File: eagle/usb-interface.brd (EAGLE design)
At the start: 18 parts

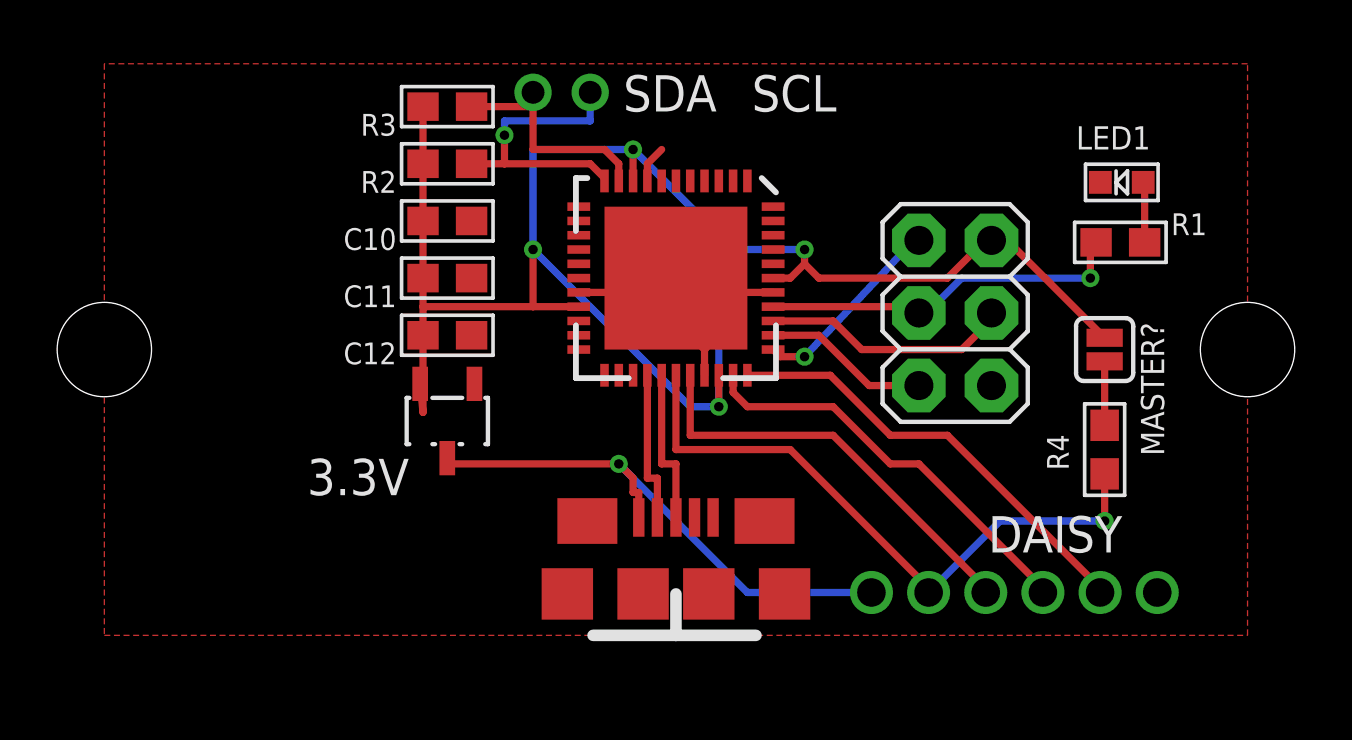
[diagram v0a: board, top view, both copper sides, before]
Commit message: major rework of usb interface board - dropped Y by 5mm, cleaned routing, added better mounting.
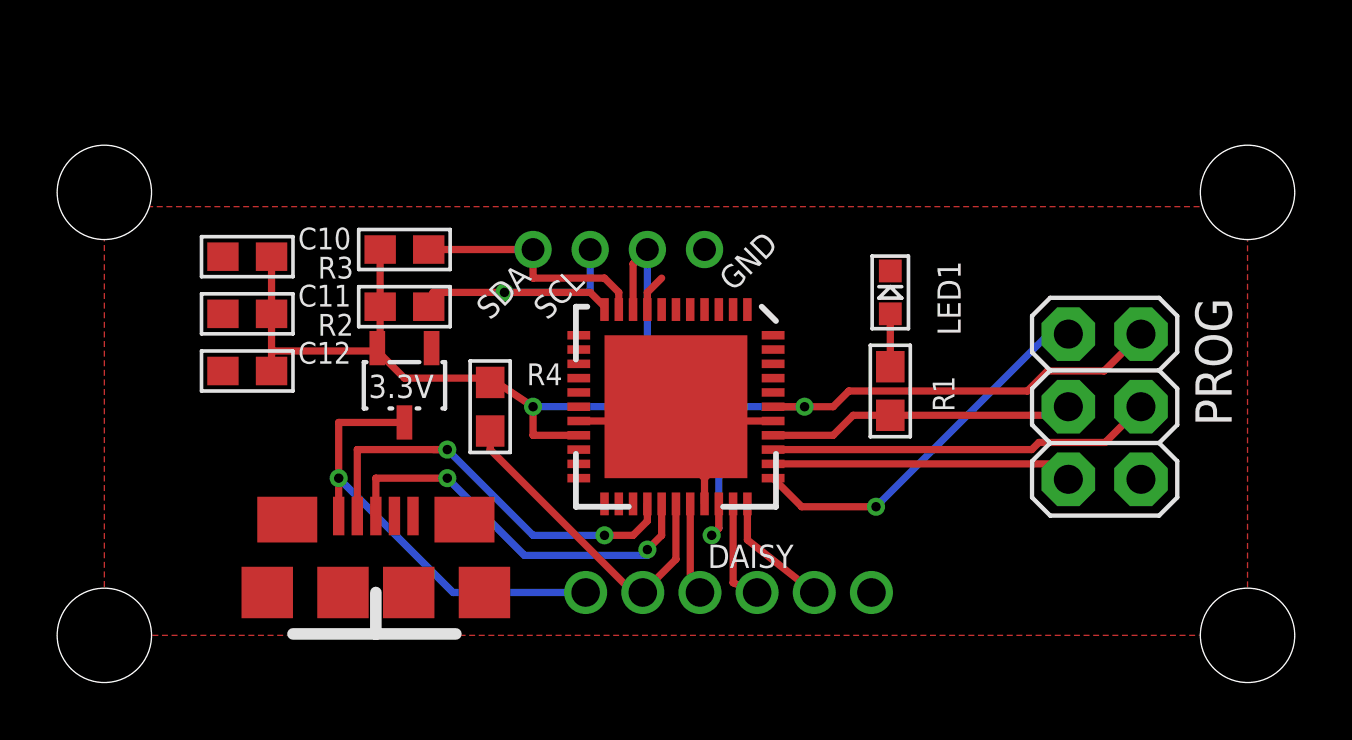
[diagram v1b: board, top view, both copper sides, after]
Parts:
- removed MASTER?: SOLDERJUMPERN, SparkFun:SJ_2S
- added JP1, JP2: (no value), nonolith:1X01_2MM
- added U$3, U$4: (no value), nonolith:STAND-OFF
- moved R4 21.6 mm to (-6.50, 8.00)
- moved CN1 10.5 mm to (-10.5, 1.50)
- moved DAISY 10.0 mm to (7.00, 1.50)
- moved U$1 10.0 mm to (-20.0, 0.00)
- moved U$2 10.0 mm to (20.0, 0.00)
- moved R1 9.58 mm to (7.50, 8.55), turned to 90 degrees
- moved LED1 8.97 mm to (7.50, 12.0), turned to 0 degrees
- moved C10 7.11 mm to (-15.0, 13.2), turned to 0 degrees
- moved C11 7.11 mm to (-15.0, 11.2), turned to 0 degrees
- moved C12 7.11 mm to (-15.0, 9.25), turned to 0 degrees
- moved PROG 6.17 mm to (15.0, 8.00)
- moved SCL 5.50 mm to (-3.00, 13.5)
- moved SDA 5.50 mm to (-5.00, 13.5)
- moved R2 5.22 mm to (-9.50, 11.5)
- moved R3 5.22 mm to (-9.50, 13.5)
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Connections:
- removed net PE0-PULL: MASTER?.2, R4.2
- net 3.3V: now also JP2.1, R4.2; no longer MASTER?.1
- net GND: now also JP1.1
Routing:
- net PE3: track 15.7 -> 4.24 mm
- net PE1: track 14.8 -> 3.64 mm
- net PE0: track 22.5 -> 11.6 mm, vias 1 -> 0
- net PE2: track 14.4 -> 3.67 mm
- net USB-: track 5.32 -> 15.0 mm, vias 0 -> 2
- net USB+: track 5.47 -> 14.0 mm, vias 0 -> 2
- net 3.3V: track 64.8 -> 57.4 mm, vias 4 -> 3
- net PDI-DATA: track 6.97 -> 13.2 mm
- net PDI-CLK: track 5.73 -> 10.8 mm
- net BOOTLOAD: track 8.73 -> 13.5 mm
- net 5V: track 19.2 -> 15.9 mm
- net PR1: track 13.5 -> 10.7 mm, vias 1 -> 0
- net PE0-PULL: track 2.24 -> 0.00 mm
- net SCL: track 10.5 -> 11.5 mm
- net SDA: track 7.96 -> 8.46 mm
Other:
- board text added: "GND"
- board text added: "SCL"
- board text added: "SDA"

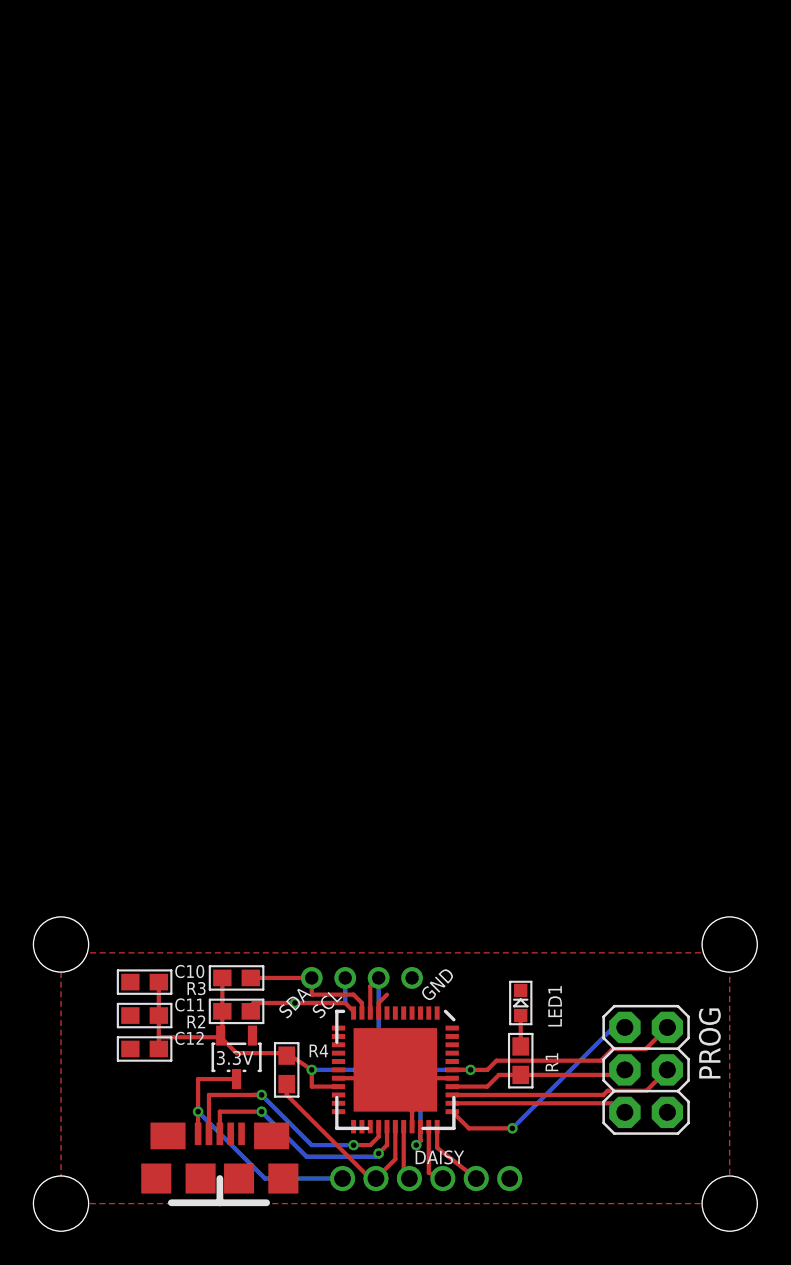
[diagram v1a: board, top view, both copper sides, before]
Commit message: reworked silkscreen and snap on tesselate.brd
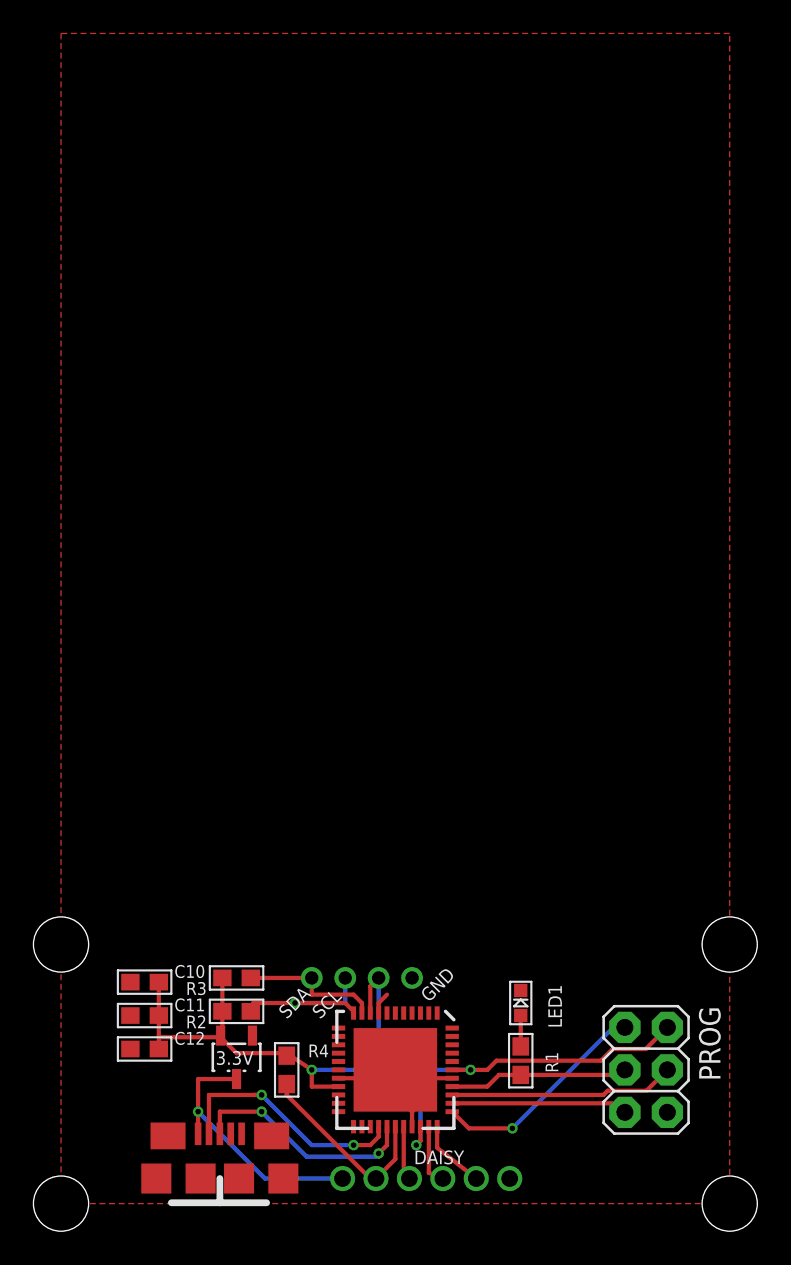
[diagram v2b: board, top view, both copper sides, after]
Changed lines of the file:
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@@
 <vertex x="-20" y="0"/>
 <vertex x="20" y="0"/>
-<vertex x="20" y="15"/>
-<vertex x="-20" y="15"/>
+<vertex x="20" y="70"/>
+<vertex x="-20" y="70"/>
 </polygon>
 <wire x1="-1" y1="11.4" x2="-1" y2="12" width="0.254" layer="1"/>

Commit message: added usb-interface from fullArray
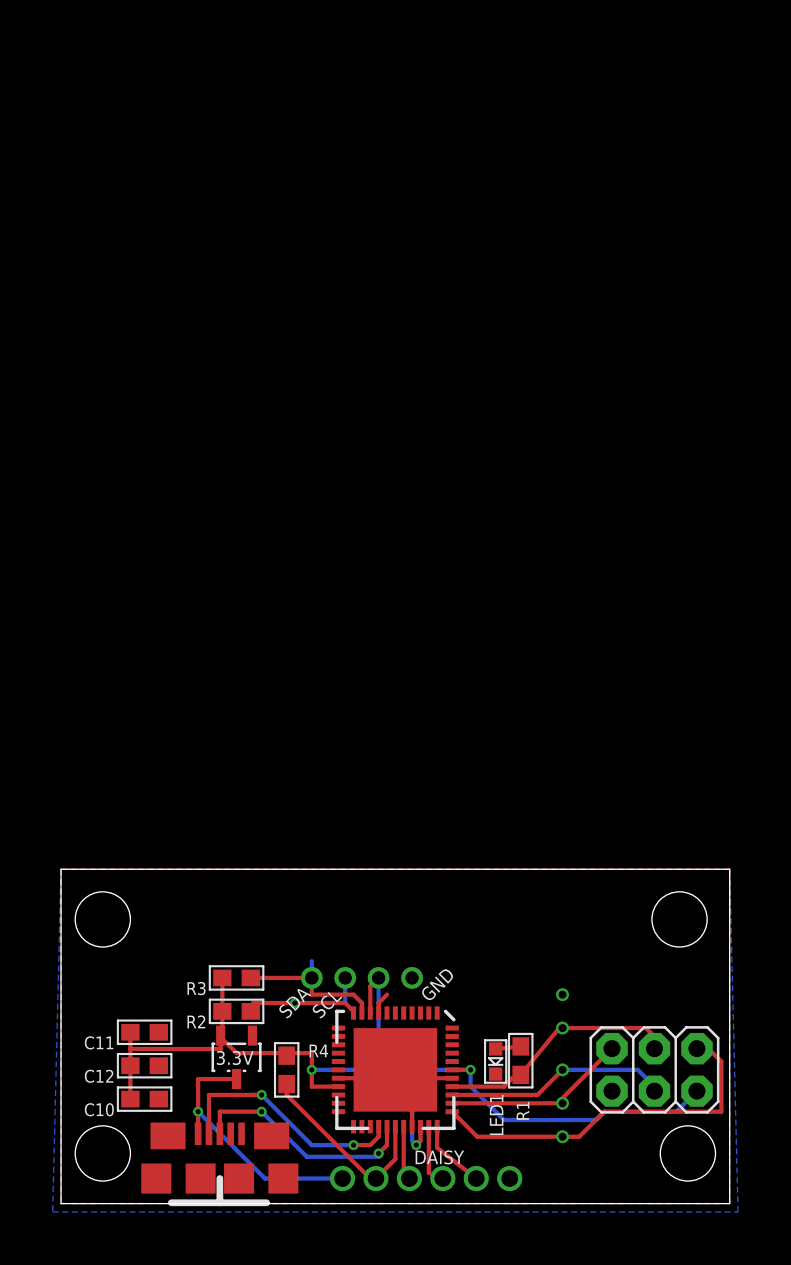
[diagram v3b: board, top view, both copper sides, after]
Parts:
- removed PROG: (no value), nonolith:2X03
- added PROGX: (no value), nonolith:2X03
- added U$5: (no value), nonolith:LOGO_NONOLITH
- R1: value (none) -> 120o
- R2, R3: value (none) -> 4.7K
- R4: value (none) -> 4.7k
- moved C10 7.00 mm to (-15.0, 6.25), turned to 180 degrees
- moved U$1 3.91 mm to (-17.5, 3.00)
- moved U$2 3.91 mm to (17.5, 3.00)
- moved LED1 3.81 mm to (6.00, 8.50), turned to 180 degrees
- moved U$4 3.35 mm to (17.0, 17.0)
- moved U$3 2.92 mm to (-17.5, 17.0)
- moved C11 1.00 mm to (-15.0, 10.2), turned to 180 degrees
- moved C12 1.00 mm to (-15.0, 8.25), turned to 180 degrees
- renumbered IC1 to XM1
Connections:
- net 3.3V: now also PROGX.2; no longer PROG.2
- net BOOTLOAD: now also PROGX.4; no longer PROG.4
- net GND: now also PROGX.6; no longer PROG.6
- net PDI-CLK: now also PROGX.5; no longer PROG.5
- net PDI-DATA: now also PROGX.1; no longer PROG.1
- net PR1: now also PROGX.3; no longer PROG.3
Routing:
- net PDI-DATA: track 13.2 -> 22.1 mm
- net 3.3V: track 57.4 -> 63.7 mm
- net PR1: track 10.7 -> 14.6 mm, vias 0 -> 1
- net SDA: track 8.46 -> 9.46 mm
- net PDI-CLK: track 10.8 -> 11.2 mm, vias 0 -> 1
- net BOOTLOAD: track 13.5 -> 13.4 mm, vias 0 -> 1
- net GND: vias 0 -> 1
- added copper zone on layer 16, net GND
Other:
- board outline added: 40 x 20 mm
